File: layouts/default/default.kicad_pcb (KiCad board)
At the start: 2 copper layers, 120 x 130 mm, 87 parts

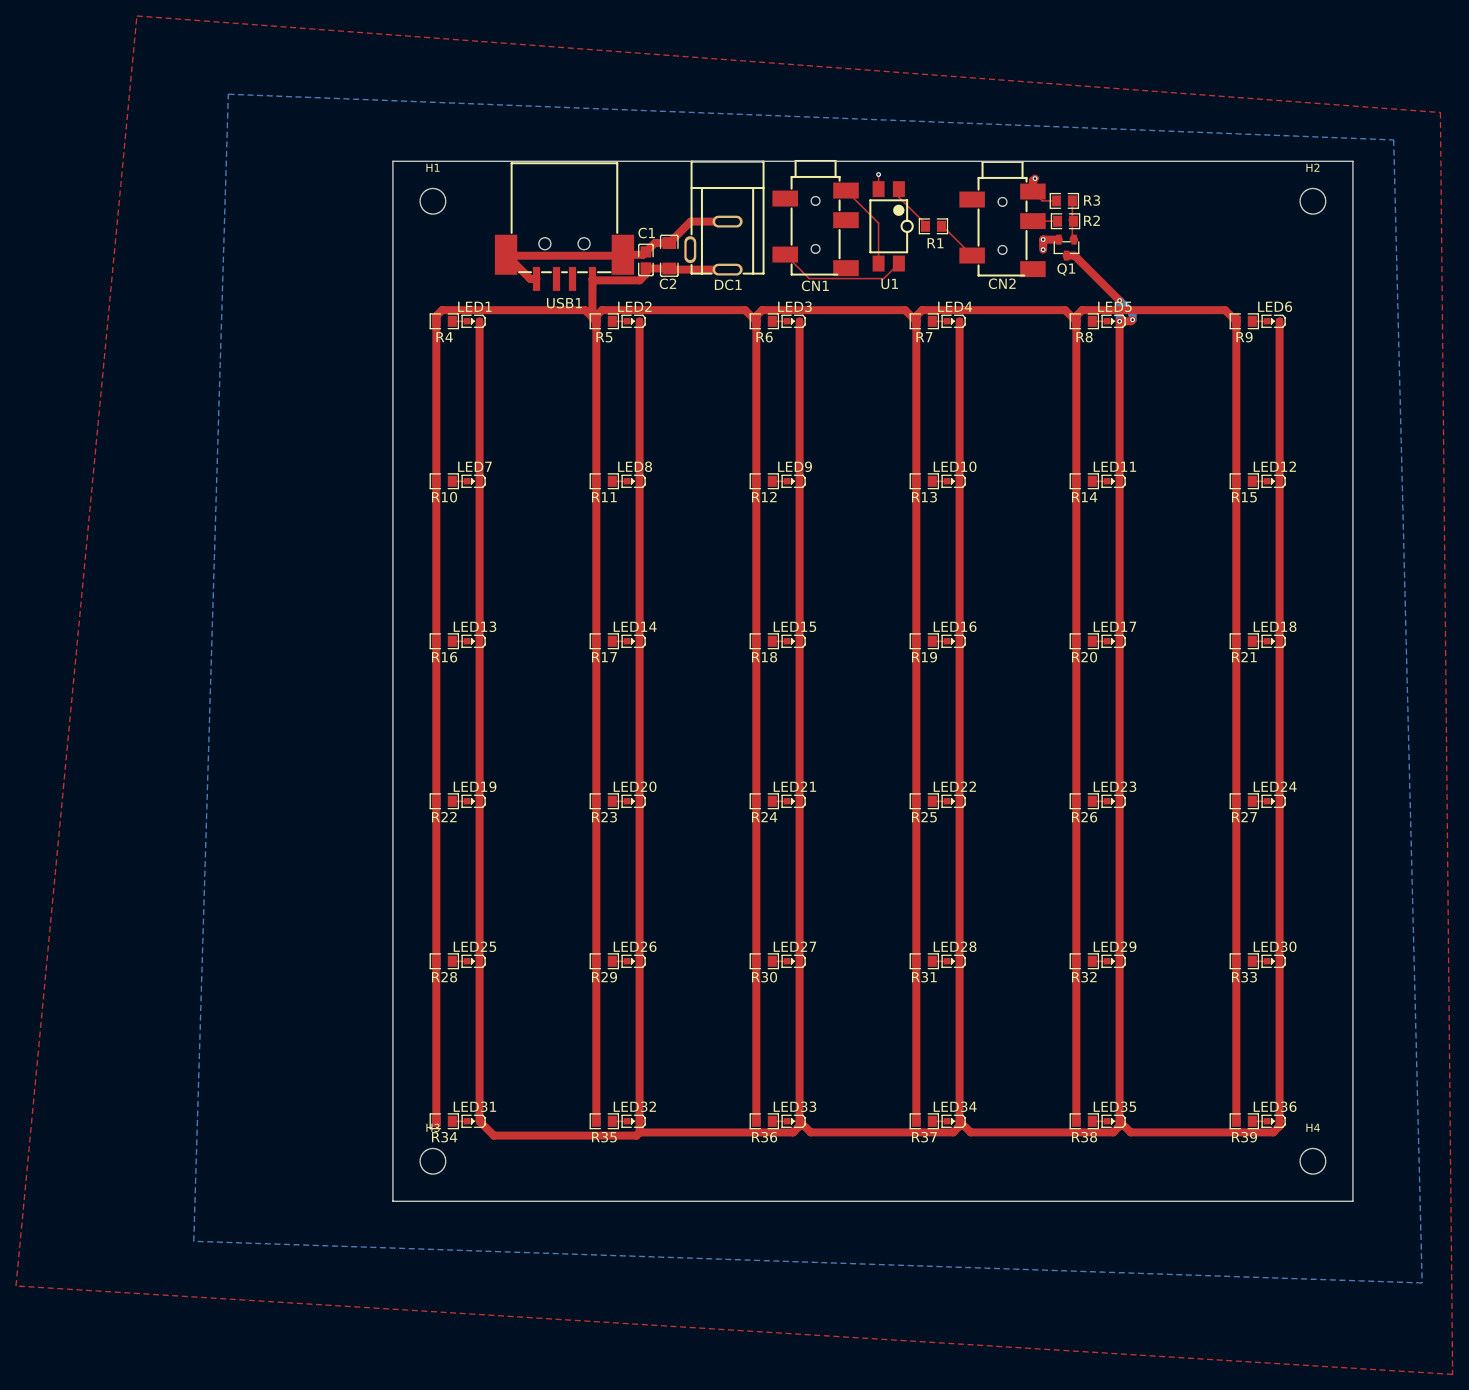
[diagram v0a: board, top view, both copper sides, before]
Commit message: done
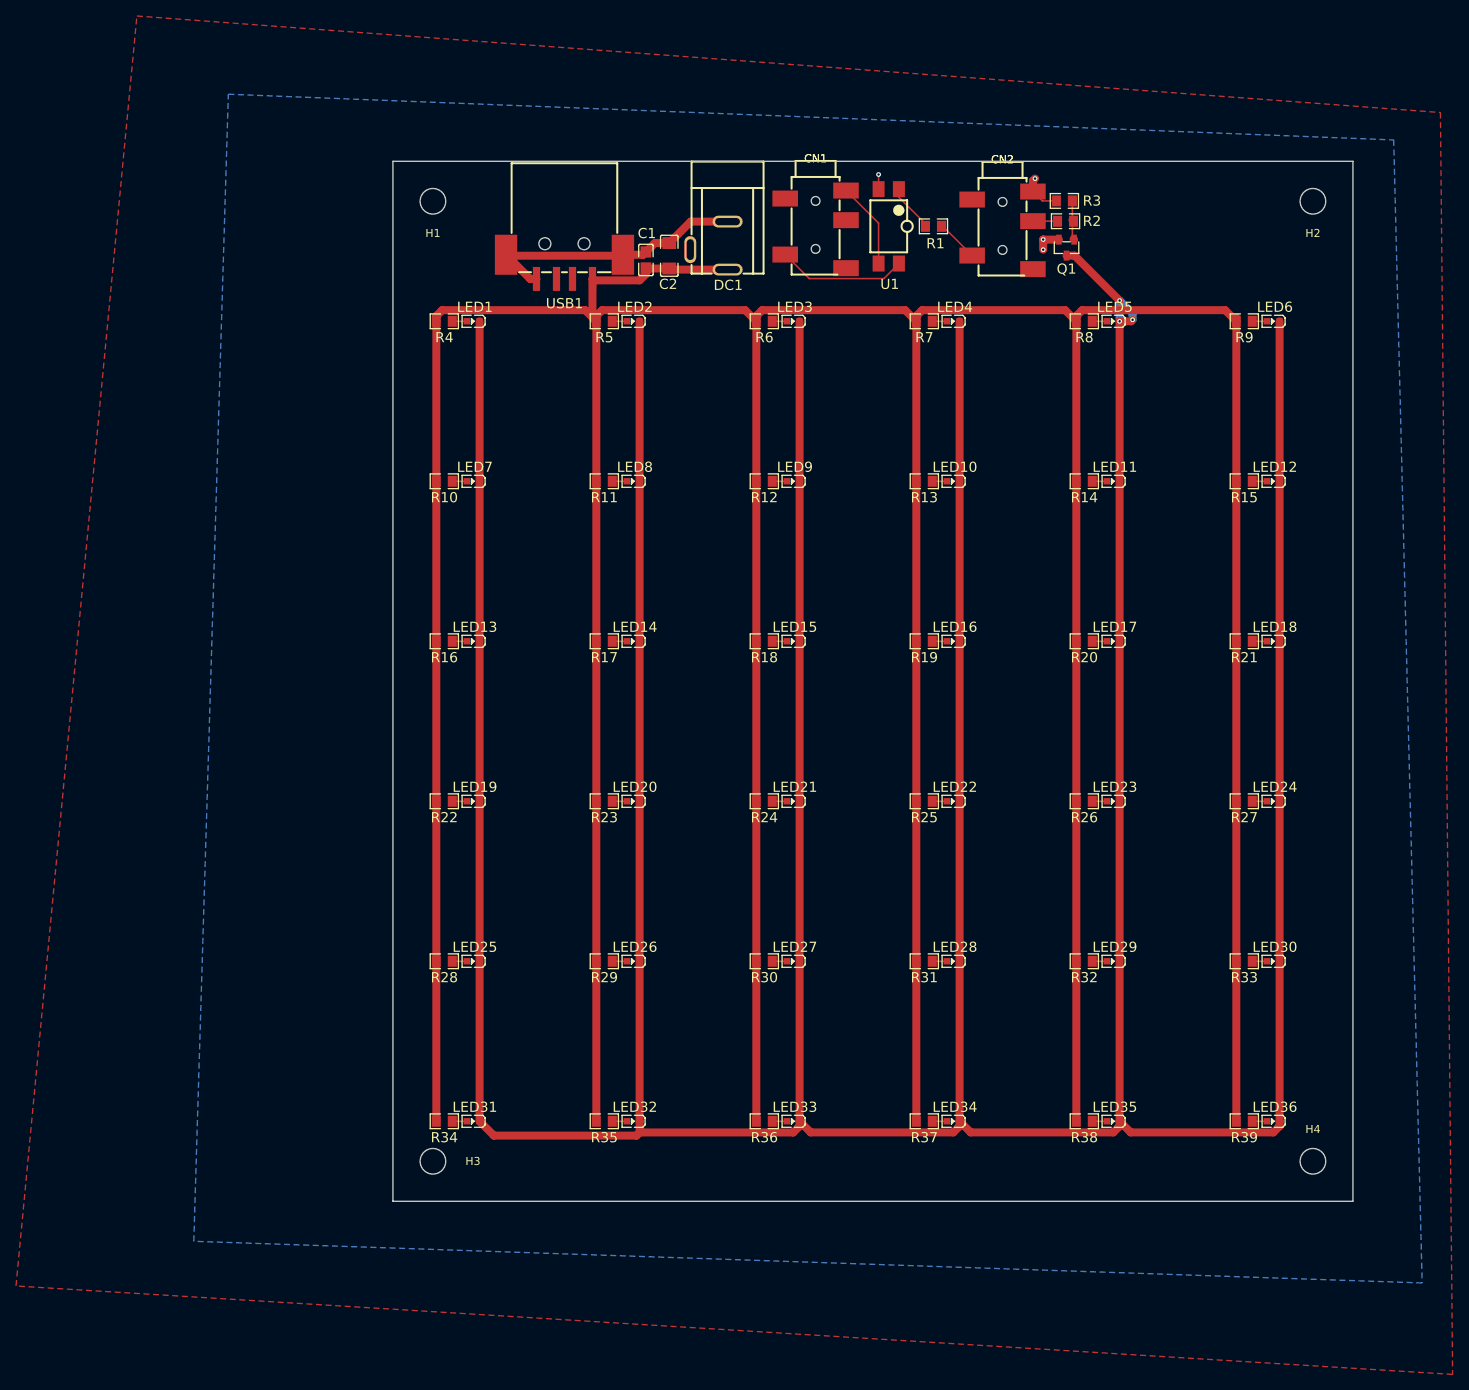
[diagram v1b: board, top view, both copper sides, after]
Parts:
- H1, H2, H3, H4: value MountingHole_3.2mm_M3 -> (none)
